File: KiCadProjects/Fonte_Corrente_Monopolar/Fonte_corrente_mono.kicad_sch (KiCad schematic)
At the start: 24 parts, among them J1 Vref, J2 tensoes, J3 sinais analogicos, J4 comunicacao / sinais digitais, J5 Vref, J6 Pinos de verificação, U1 AD828AN, U2 INA128, U3 AD828AN

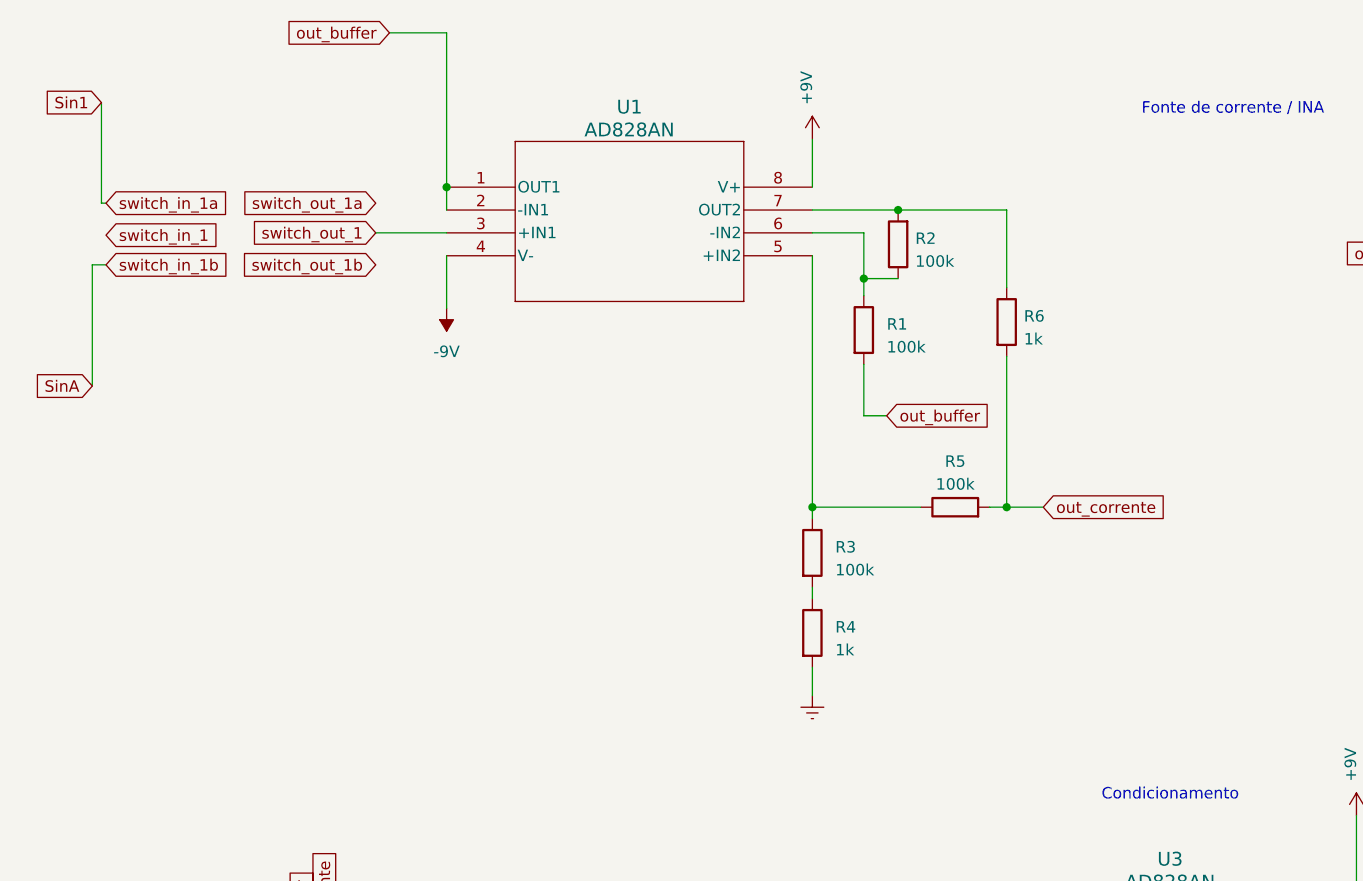
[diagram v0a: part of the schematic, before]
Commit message: autosave backup
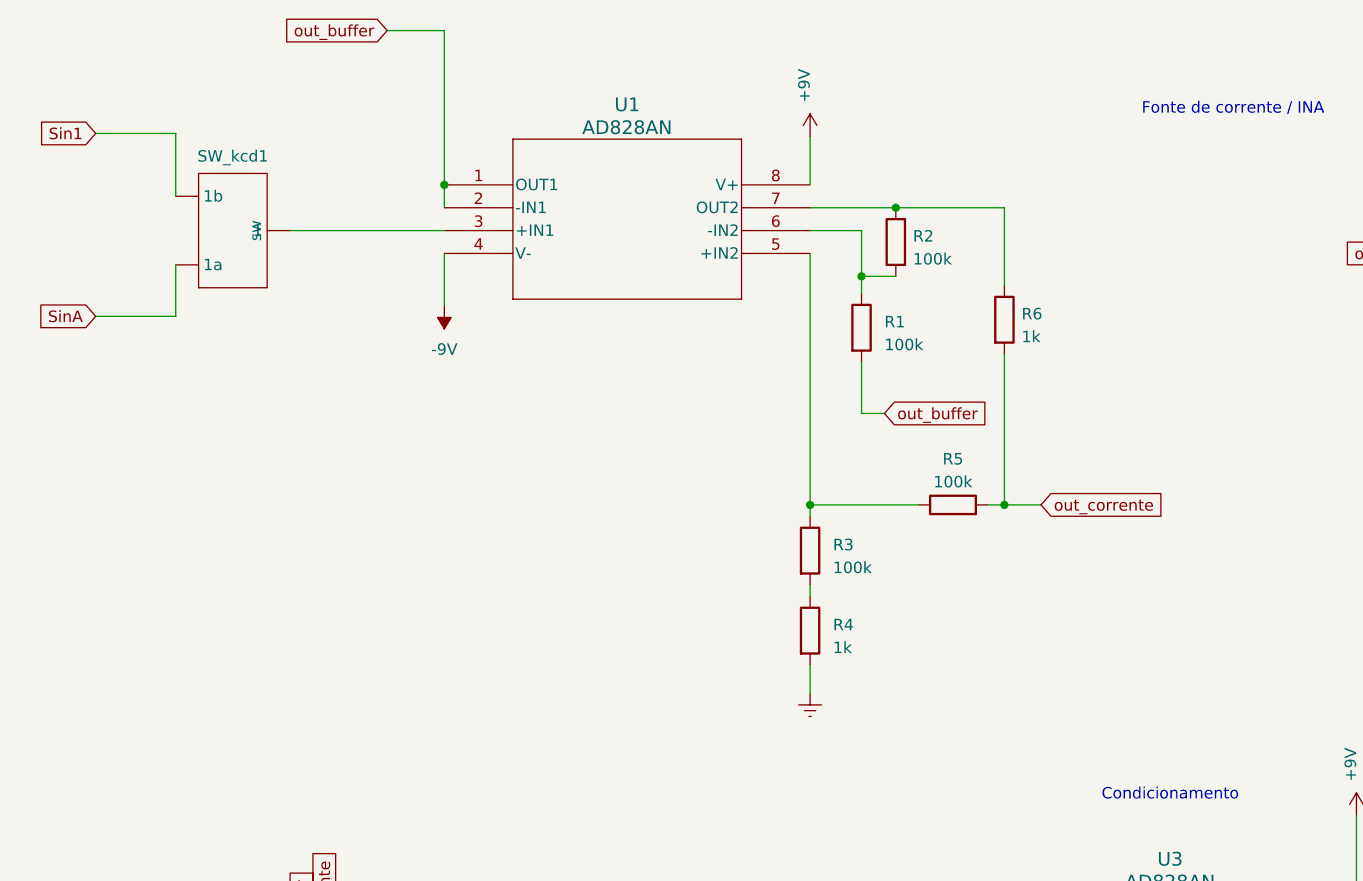
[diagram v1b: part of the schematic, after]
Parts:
- added SW_kcd1: sw, Chave_Gangorra:chave gangorra 3 pinos, symbol chave_gangorra_kcd1_2pinos:chave_gangorra_
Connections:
- net Sin1: now also SW_kcd1. (1a)
- net SinA: now also SW_kcd1. (1a)
- net switch_out_1: no longer names the net of U1.3 (+IN1)
- net switch_out_1: now also SW_kcd1. (1a)

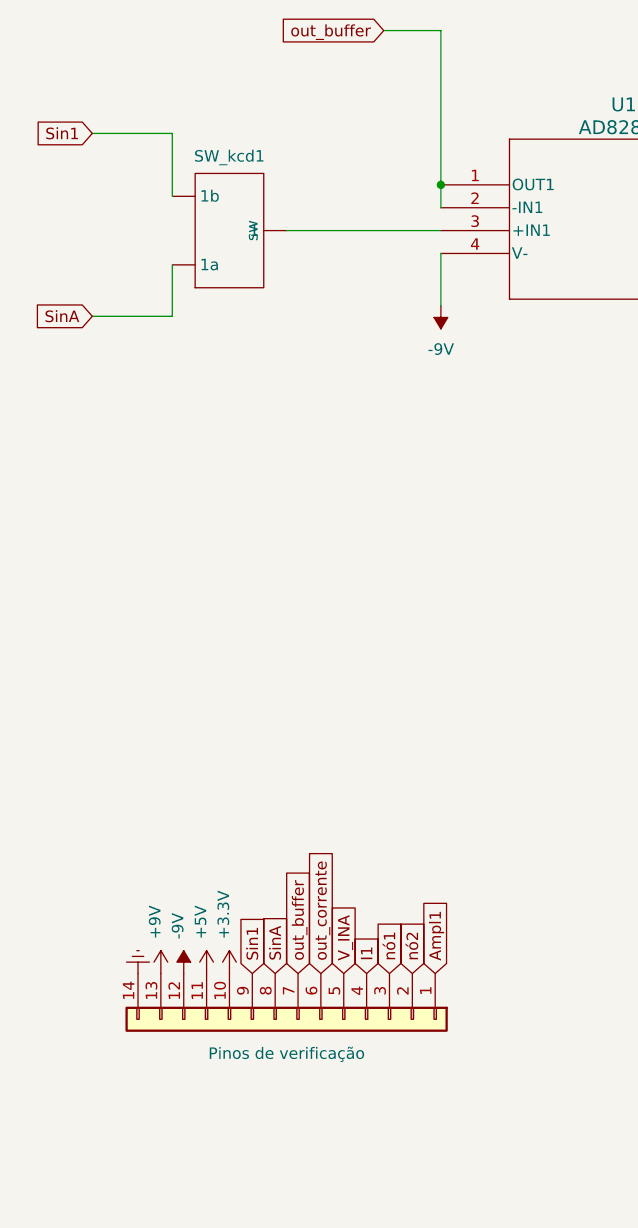
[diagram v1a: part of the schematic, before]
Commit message: alterações PCB
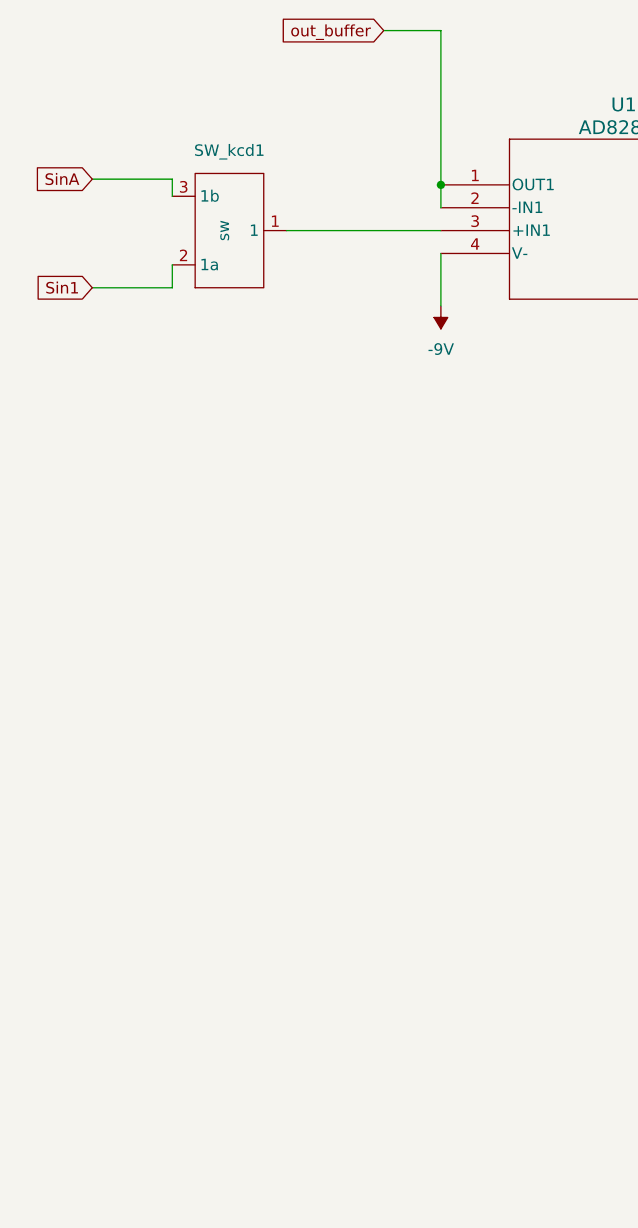
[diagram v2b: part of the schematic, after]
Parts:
- removed J6: Pinos de verificação, Connector_PinHeader_2.54mm:PinHeader_1x14_P2.54mm_Horizontal, symbol Connector_Generic:Conn_01x14
- removed SW_kcd1: sw, Chave_Gangorra:chave gangorra 3 pinos, symbol chave_gangorra_kcd1_2pinos:chave_gangorra_
- added SW_kcd1: sw, Chave_Gangorra:chave gangorra 3 pinos, symbol chave_gangorra_kcd1:chave_gangorra_
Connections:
- net Sin1: now also SW_kcd1.2 (1a)
- net SinA: now also SW_kcd1.3 (1b)
- net at U1.3 (+IN1): now also SW_kcd1.1

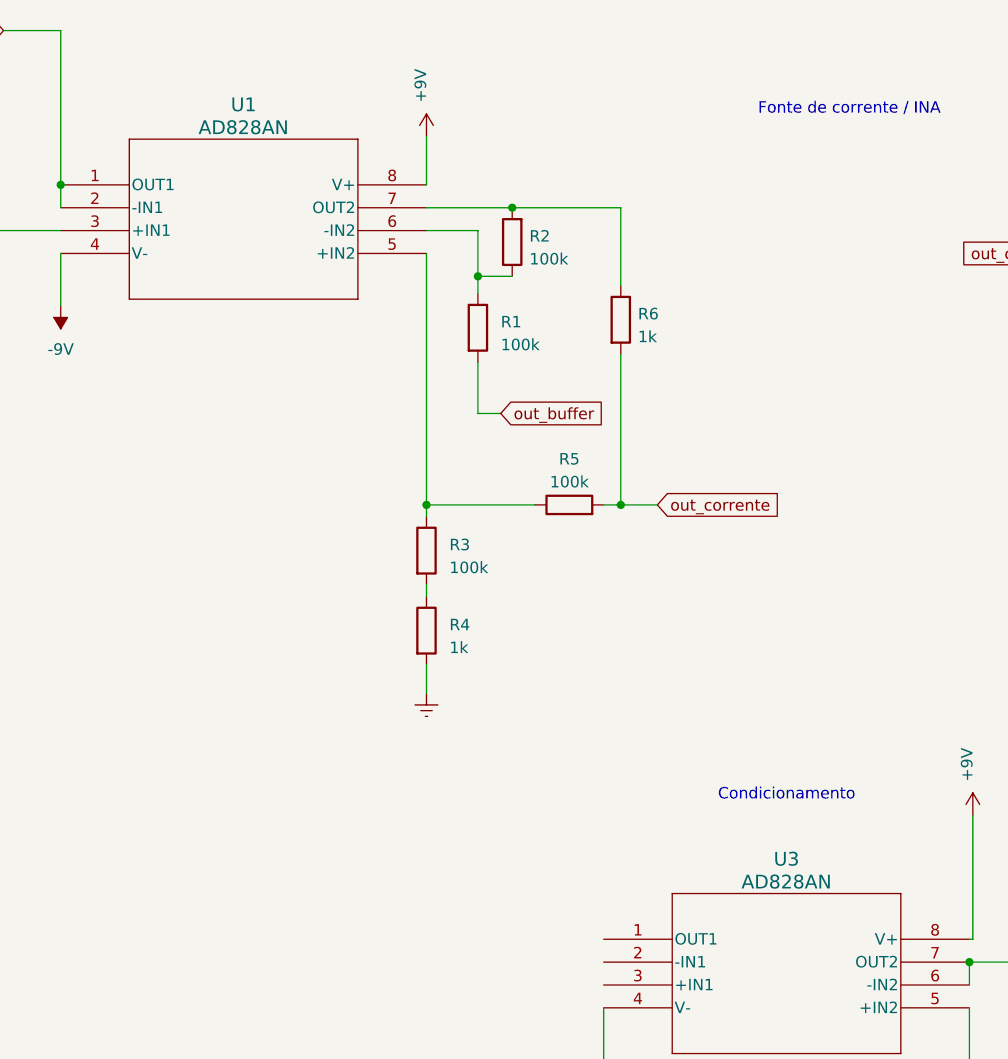
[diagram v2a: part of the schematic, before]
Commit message: alterações PCB
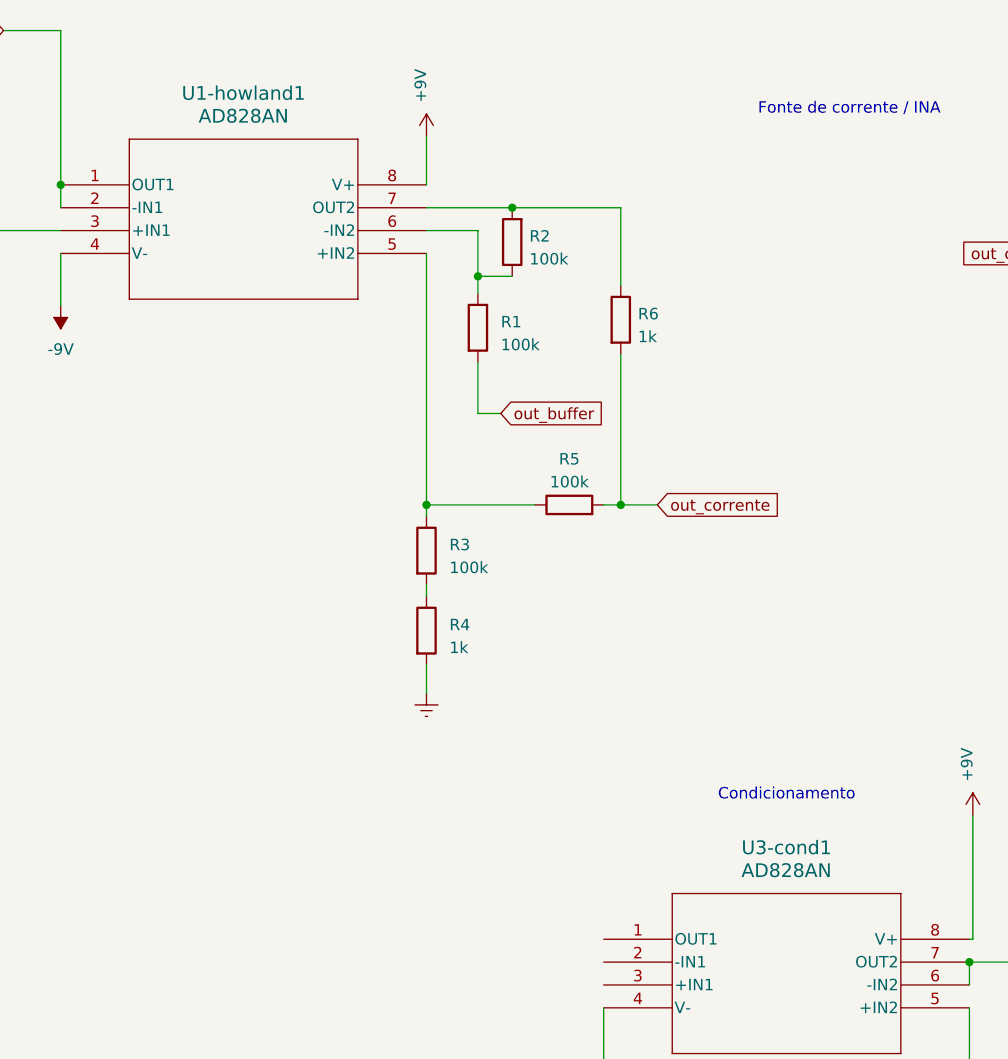
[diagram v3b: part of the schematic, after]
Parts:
- renumbered U1 to U1-howland1, U3 to U3-cond1
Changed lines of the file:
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@@
   (symbol (lib_id "AD828AN:AD828AN") (at 118.745 116.84 0) (unit 1)
     (in_bom yes) (on_board yes) (dnp no) (fields_autoplaced)
-    (property "Reference" "U3" (at 139.065 107.95 0)
+    (property "Reference" "U3-cond1" (at 139.065 106.68 0)
       (effects (font (size 1.524 1.524)))
     )
-    (property "Value" "AD828AN" (at 139.065 110.49 0)
+    (property "Value" "AD828AN" (at 139.065 109.22 0)
       (effects (font (size 1.524 1.524)))
     )
@@
       (project "Fonte_corrente_mono"
         (path "/f0ff92cf-26e5-4ab9-977d-5f9689e8a5d0"
-          (reference "U3") (unit 1)
+          (reference "U3-cond1") (unit 1)
         )
       )
@@
   (symbol (lib_id "2023-04-18_19-29-20:AD828AN") (at 58.42 33.02 0) (unit 1)
     (in_bom yes) (on_board yes) (dnp no) (fields_autoplaced)
-    (property "Reference" "U1" (at 78.74 24.13 0)
+    (property "Reference" "U1-howland1" (at 78.74 22.86 0)
       (effects (font (size 1.524 1.524)))
     )
-    (property "Value" "AD828AN" (at 78.74 26.67 0)
+    (property "Value" "AD828AN" (at 78.74 25.4 0)
       (effects (font (size 1.524 1.524)))
     )
@@
       (project "Fonte_corrente_mono"
         (path "/f0ff92cf-26e5-4ab9-977d-5f9689e8a5d0"
-          (reference "U1") (unit 1)
-        )
-      )
+          (reference "U1-howland1") (unit 1)
+        )
+      )
